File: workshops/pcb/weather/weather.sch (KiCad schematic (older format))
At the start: 9 parts, among them J1 Barrel_Jack, J2 Conn_01x04_Female, J3 Conn_01x03_Female, J4 Conn_01x03_Female, J5 Conn_01x08_Female, J6 Conn_01x01_Female, J7 Conn_01x02_Female, J8 Conn_01x05_Female, U1 ESP8266NodeMCU

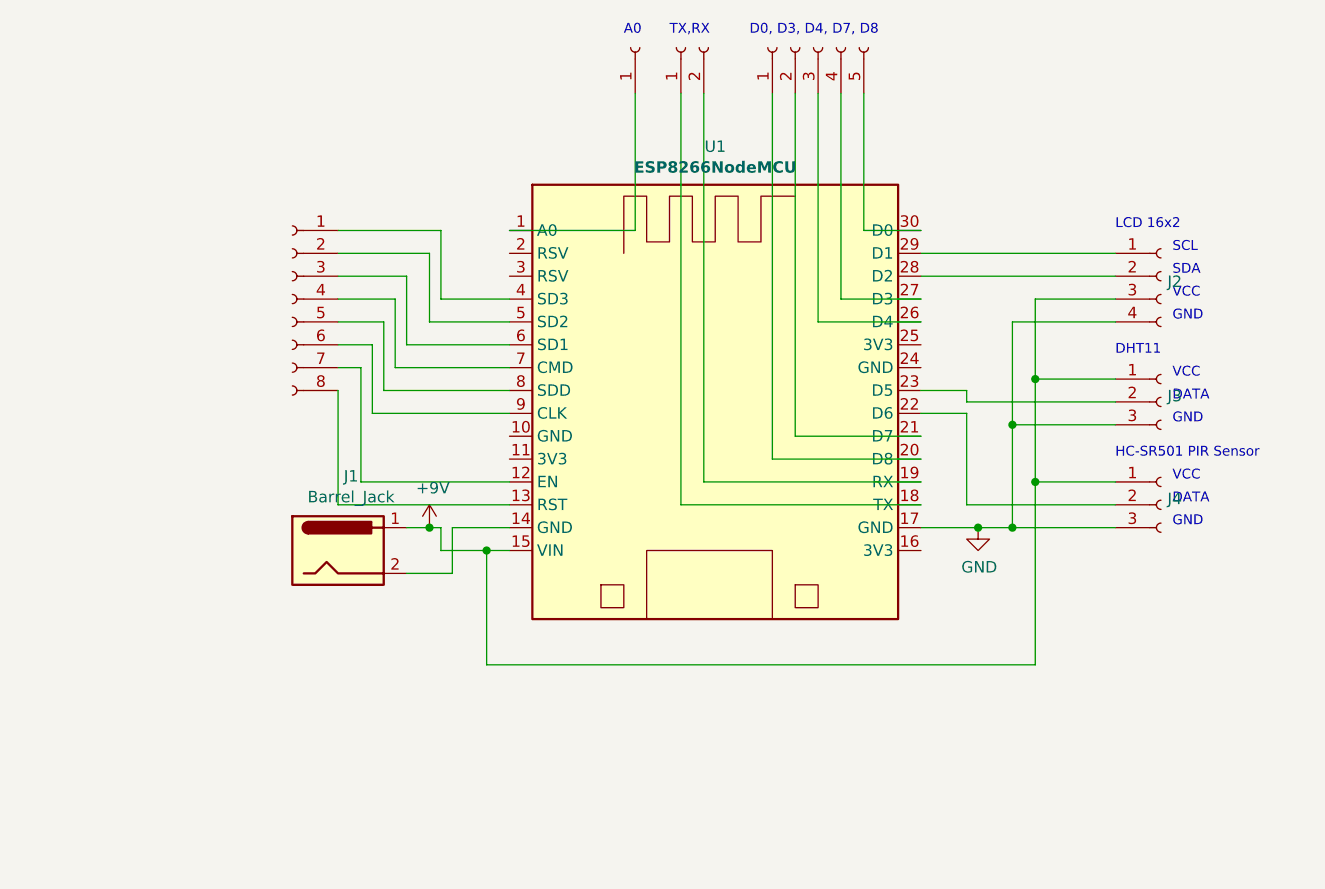
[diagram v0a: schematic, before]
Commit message: Update custom_logo.kicad_mod, fp-info-cache, and 7 more files...
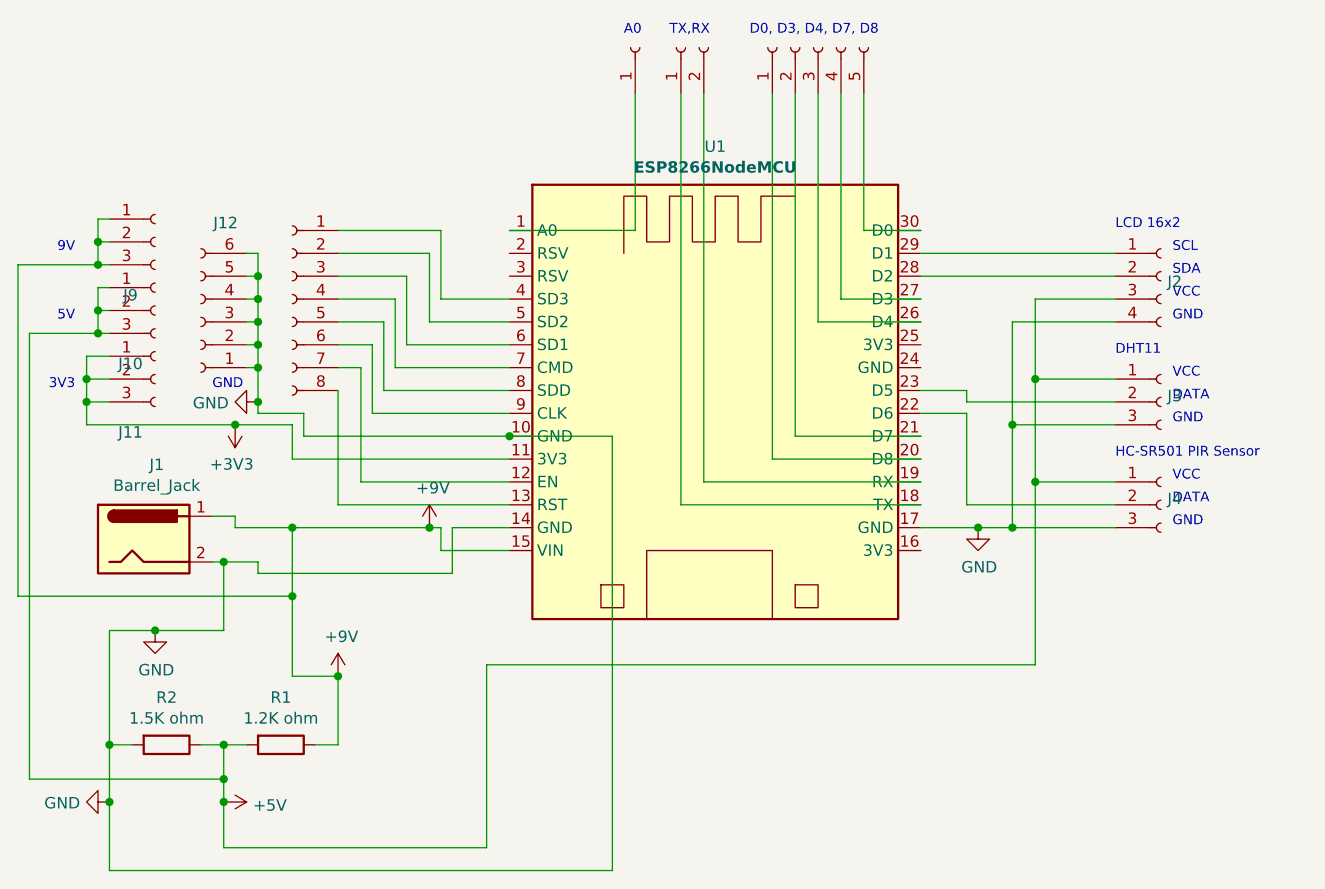
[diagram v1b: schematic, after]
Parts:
- added J10, J11, J9: Conn_01x03_Female, Connector_PinHeader_2.54mm:PinHeader_1x03_P2.54mm_Vertical, symbol Connector:Conn_01x03_Female
- added J12: Conn_01x06_Female, Connector_PinHeader_2.54mm:PinHeader_1x06_P2.54mm_Vertical, symbol Connector:Conn_01x06_Female
- added R1: 1.2K ohm, Resistor_THT:R_Axial_DIN0309_L9.0mm_D3.2mm_P12.70mm_Horizontal, symbol Device:R
- added R2: 1.5K ohm, Resistor_THT:R_Axial_DIN0309_L9.0mm_D3.2mm_P12.70mm_Horizontal, symbol Device:R
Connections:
- net +9V: now also J9.1 (Pin_1), J9.2 (Pin_2), J9.3 (Pin_3), R1.1; no longer J2.3 (Pin_3), J3.1 (Pin_1), J4.1 (Pin_1)
- net GND: now also J1.2, U1.10 (GND), U1.14 (GND), J12.1 (Pin_1), J12.2 (Pin_2), J12.3 (Pin_3), J12.4 (Pin_4), J12.5 (Pin_5), J12.6 (Pin_6), R2.2
- net +3V3: now reaches U1.11 (3V3)
- net +3V3: now also J11.1 (Pin_1), J11.2 (Pin_2), J11.3 (Pin_3)
- new net +5V: J10.1 (Pin_1), J10.2 (Pin_2), J10.3 (Pin_3), J2.3 (Pin_3), J3.1 (Pin_1), J4.1 (Pin_1), R1.2, R2.1
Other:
- note added: "3V3"
- note added: "5V"
- note added: "9V"
- moved on the sheet: J1
